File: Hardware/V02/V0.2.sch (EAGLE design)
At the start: 32 parts, among them IC101 ADS124S06IPBS, X101 MOLEX-8738-0343, X102 A97581-ND, X103 A97581-ND, X104 A97581-ND, X105 33PIN-2.54

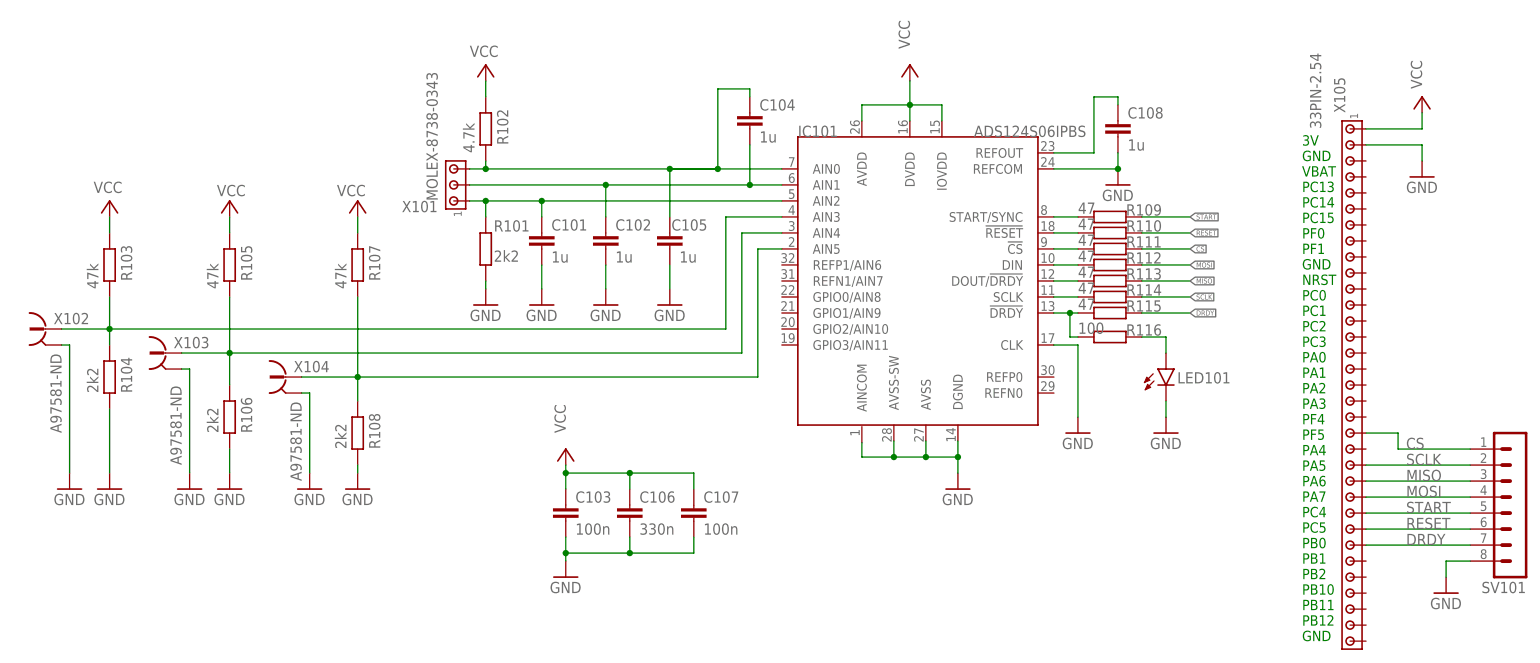
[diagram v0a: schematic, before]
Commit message: Schemaänderung; BNC-Abschwächer
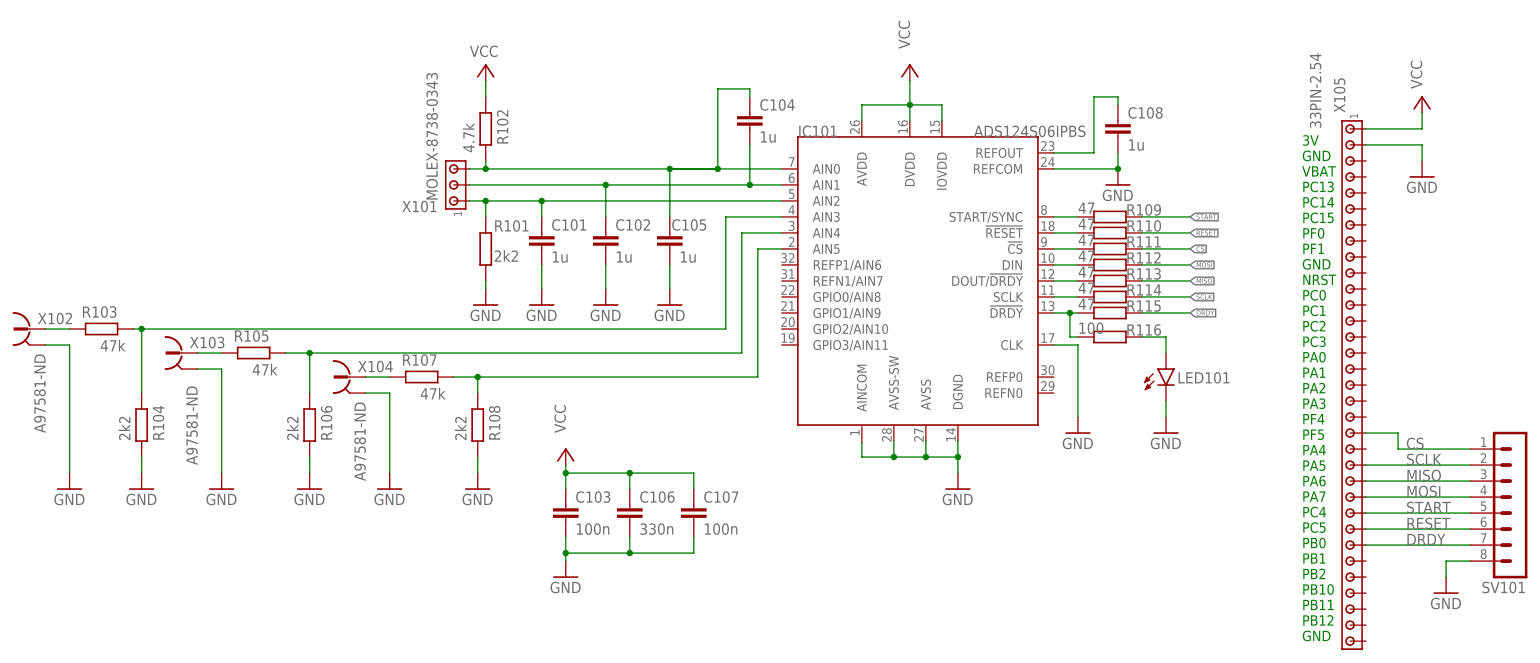
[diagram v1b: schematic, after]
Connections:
- new net N$12: R103.2, X102.1
- new net N$13: R105.2, X103.1
- new net N$16: R107.2, X104.1
- net N$11: no longer X102.1
- net N$17: no longer X103.1
- net N$18: no longer X104.1
- net VCC: no longer R103.2, R105.2, R107.2
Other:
- moved on the sheet: R103, R104, R105, R106, R107, R108, X102, X103, X104
